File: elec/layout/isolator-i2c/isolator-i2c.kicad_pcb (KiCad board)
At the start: 2 copper layers, 7 parts, among them U1 10kΩ ±1% 62.5mW, U2 10kΩ ±1% 62.5mW, U4 10kΩ ±1% 62.5mW, U5 10kΩ ±1% 62.5mW, U6 100nF ±10% 16V X7R, U7 100nF ±10% 16V X7R

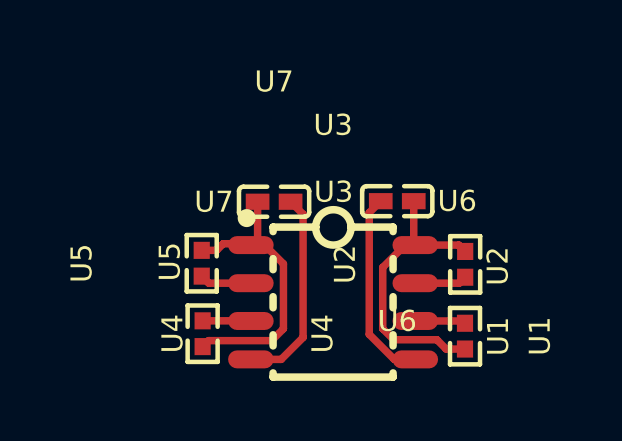
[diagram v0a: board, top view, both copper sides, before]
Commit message: Everything builds
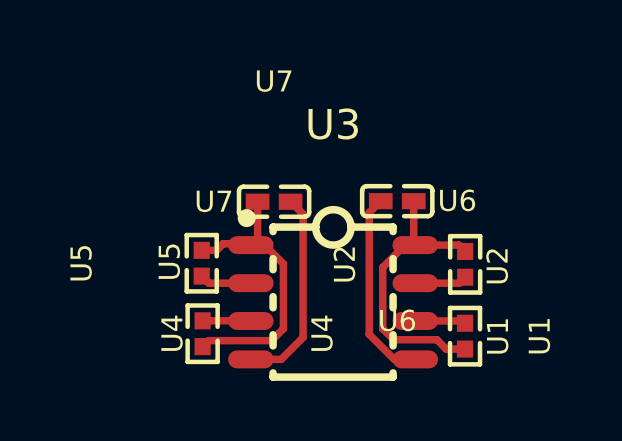
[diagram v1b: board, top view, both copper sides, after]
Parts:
- U1, U2, U4, U5: value 10kΩ ±1% 62.5mW -> 1kΩ ±1% 62.5mW
- U3: footprint lib:SOIC-8_L4.9-W3.9-P1.27-LS6.0-TL -> atopile:SOIC-8_L4.9-W3.9-P1.27-LS6.0-TL-e13595
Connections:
- U1 pad 1: line-2 -> line-1
- U1 pad 2: hv-1 -> hv
- U2 pad 2: hv-1 -> hv
- U3 pad 1: hv -> hv-1
- U3 pad 2: line-1 -> line-2
- U3 pad 6: line-2 -> line-1
- U3 pad 8: hv-1 -> hv
- U4 pad 2: hv -> hv-1
- U5 pad 1: line-1 -> line-2
- U5 pad 2: hv -> hv-1
- U6 pad 1: hv-1 -> hv
- U7 pad 1: hv -> hv-1
